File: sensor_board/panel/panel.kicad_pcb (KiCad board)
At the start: 2 copper layers, 102.6 x 93.3 mm, 165 parts, among them J1 Comm, J2 OUTPUT, J3 INPUT, J4 LDO_GND, J5 LDO_VCC, U1 INA228, U2 AMS1117/WL9005P3

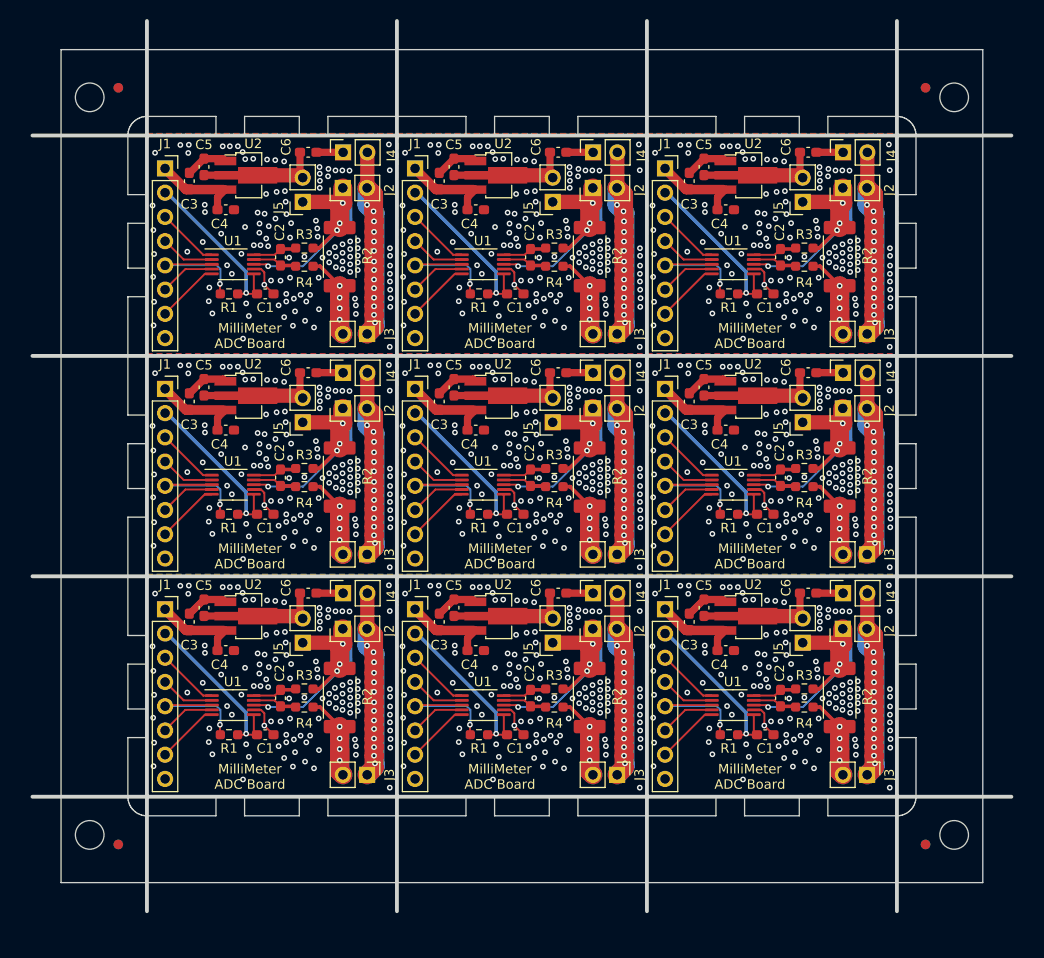
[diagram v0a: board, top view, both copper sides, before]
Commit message: Generate Rev. 1 gerber
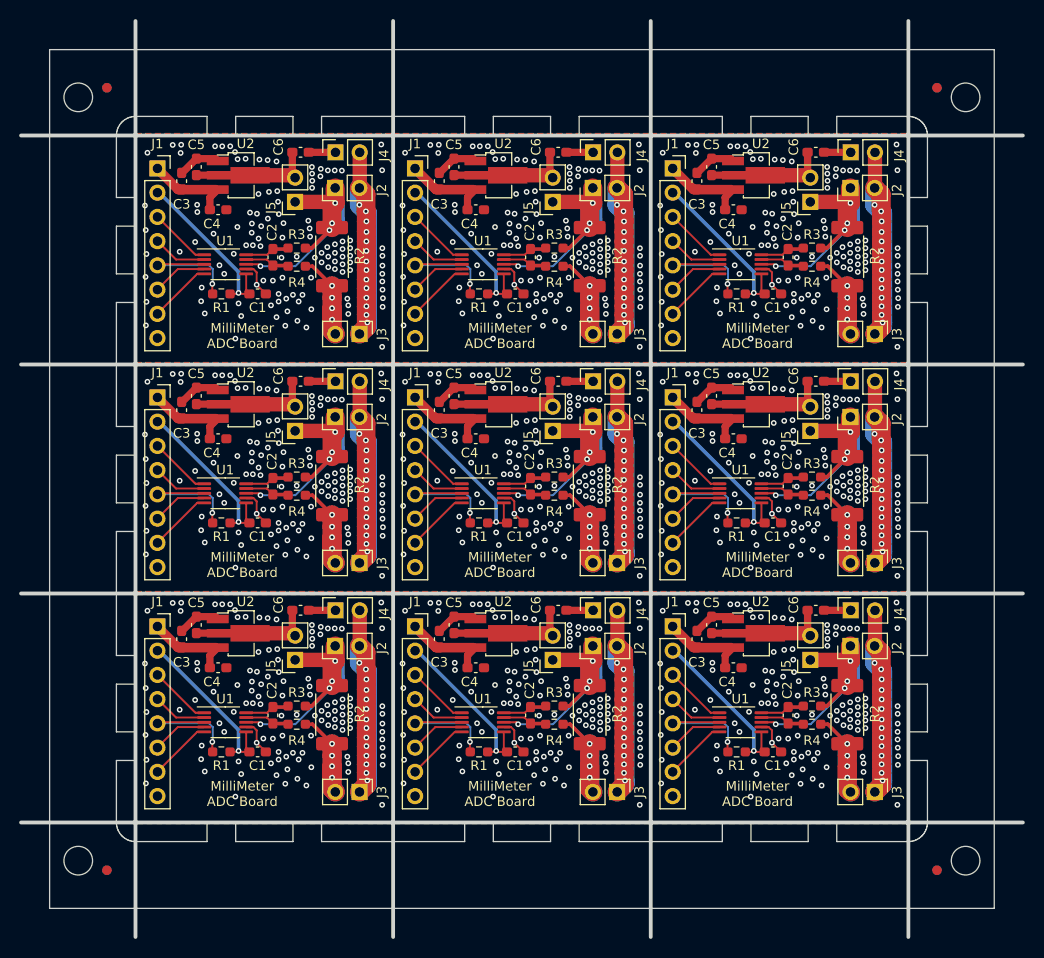
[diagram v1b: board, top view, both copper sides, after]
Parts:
- removed the C1 at (147.8, 68.7)
- removed the C1 at (121.6, 68.7)
- removed the C1 at (174.0, 91.8)
- removed the C1 at (174.0, 45.6)
- removed the C1 at (121.6, 91.8)
- removed the C1 at (121.6, 45.6)
- removed the C1 at (174.0, 68.7)
- removed the C1 at (147.8, 91.8)
- removed the C2 at (175.6, 88.0)
- removed the C2 at (149.4, 64.9)
- removed the C2 at (175.6, 41.8)
- removed the C2 at (175.6, 64.9)
- removed the C2 at (149.4, 88.0)
- removed the C2 at (123.2, 88.0)
- removed the C2 at (123.2, 64.9)
- removed the C2 at (123.2, 41.8)
- removed the C3 at (113.6, 80.0)
- removed the C3 at (139.8, 56.9)
- removed the C3 at (166.0, 56.9)
- removed the C3 at (113.6, 33.8)
- removed the C3 at (139.8, 80.0)
- removed the C3 at (166.0, 33.8)
- removed the C3 at (166.0, 80.0)
- removed the C3 at (113.6, 56.9)
- removed the C4 at (169.9, 59.9)
- removed the C4 at (143.7, 59.9)
- removed the C4 at (143.7, 83.0)
- removed the C4 at (117.5, 83.0)
- removed the C4 at (117.5, 59.9)
- removed the C4 at (117.5, 36.8)
- removed the C4 at (169.9, 36.8)
- removed the C4 at (169.9, 83.0)
- removed the C5 at (115.2, 78.5)
- removed the C5 at (167.6, 78.5)
- removed the C5 at (167.6, 55.4)
- removed the C5 at (141.4, 55.4)
- removed the C5 at (167.6, 32.3)
- removed the C5 at (141.4, 78.5)
- removed the C5 at (115.2, 32.3)
- removed the C5 at (115.2, 55.4)
- removed the C6 at (152.3, 53.9)
- removed the C6 at (178.5, 30.8)
- removed the C6 at (152.3, 77.0)
- removed the C6 at (178.5, 77.0)
- removed the C6 at (126.1, 77.0)
- removed the C6 at (126.1, 30.8)
- removed the C6 at (126.1, 53.9)
- removed the C6 at (178.5, 53.9)
- removed the J1 at (163.5, 78.7)
- removed the J1 at (111.1, 78.7)
- removed the J1 at (137.3, 78.7)
- removed the J1 at (137.3, 55.6)
- removed the J1 at (163.5, 55.6)
- removed the J1 at (111.1, 32.5)
- removed the J1 at (111.1, 55.6)
- removed the J1 at (163.5, 32.5)
- removed the J2 at (129.7, 80.7)
- removed the J2 at (182.1, 80.7)
- removed the J2 at (182.1, 57.6)
- removed the J2 at (155.9, 57.6)
- removed the J2 at (155.9, 80.7)
- removed the J2 at (129.7, 34.5)
- removed the J2 at (129.7, 57.6)
- removed the J2 at (182.1, 34.5)
- removed the J3 at (132.3, 72.9)
- removed the J3 at (184.7, 96.0)
- removed the J3 at (132.3, 96.0)
- removed the J3 at (132.3, 49.8)
- removed the J3 at (184.7, 72.9)
- removed the J3 at (158.5, 72.9)
- removed the J3 at (158.5, 96.0)
- removed the J3 at (184.7, 49.8)
- removed the J4 at (129.8, 53.9)
- removed the J4 at (182.2, 30.8)
- removed the J4 at (129.8, 77.0)
- removed the J4 at (129.8, 30.8)
- removed the J4 at (182.2, 77.0)
- removed the J4 at (156.0, 53.9)
- removed the J4 at (182.2, 53.9)
- removed the J4 at (156.0, 77.0)
- removed the J5 at (125.5, 82.2)
- removed the J5 at (125.5, 59.1)
- removed the J5 at (151.7, 82.2)
- removed the J5 at (177.9, 82.2)
- removed the J5 at (177.9, 36.0)
- removed the J5 at (151.7, 59.1)
- removed the J5 at (177.9, 59.1)
- removed the J5 at (125.5, 36.0)
- removed the R1 at (170.2, 91.8)
- removed the R1 at (117.8, 45.6)
- removed the R1 at (117.8, 68.7)
- removed the R1 at (117.8, 91.8)
- removed the R1 at (170.2, 68.7)
- removed the R1 at (170.2, 45.6)
- removed the R1 at (144.0, 91.8)
- removed the R1 at (144.0, 68.7)
- removed the R2 at (129.4, 41.7)
- removed the R2 at (181.8, 87.9)
- removed the R2 at (129.4, 87.9)
- removed the R2 at (181.8, 41.7)
- removed the R2 at (181.8, 64.8)
- removed the R2 at (155.6, 87.9)
- removed the R2 at (129.4, 64.8)
- removed the R2 at (155.6, 64.8)
- removed the R3 at (151.9, 87.0)
- removed the R3 at (125.7, 63.9)
- removed the R3 at (178.1, 40.8)
- removed the R3 at (178.1, 87.0)
- removed the R3 at (151.9, 63.9)
- removed the R3 at (178.1, 63.9)
- removed the R3 at (125.7, 87.0)
- removed the R3 at (125.7, 40.8)
- removed the R4 at (178.1, 88.9)
- removed the R4 at (125.7, 42.7)
- removed the R4 at (125.7, 88.9)
- removed the R4 at (151.9, 88.9)
- removed the R4 at (151.9, 65.8)
- removed the R4 at (178.1, 65.8)
- removed the R4 at (125.7, 65.8)
- removed the R4 at (178.1, 42.7)
- removed the REF** at (103.2, 25.0)
- removed the REF** at (106.2, 103.3) (x2)
- removed the REF** at (106.2, 24.0) (x2)
- removed the REF** at (190.8, 24.0) (x2)
- removed the REF** at (193.8, 102.3)
- removed the REF** at (193.8, 25.0)
- removed the REF** at (190.8, 103.3) (x2)
- removed the REF** at (103.2, 102.3)
- removed the U1 at (144.4, 65.6)
- removed the U1 at (118.2, 65.6)
- removed the U1 at (170.6, 42.5)
- removed the U1 at (170.6, 88.7)
- removed the U1 at (118.2, 88.7)
- removed the U1 at (118.2, 42.5)
- removed the U1 at (144.4, 88.7)
- removed the U1 at (170.6, 65.6)
- removed the U2 at (145.8, 56.3)
- removed the U2 at (172.0, 33.2)
- removed the U2 at (119.6, 56.3)
- removed the U2 at (145.8, 79.4)
- removed the U2 at (172.0, 56.3)
- removed the U2 at (119.6, 79.4)
- removed the U2 at (119.6, 33.2)
- removed the U2 at (172.0, 79.4)
- added C1: 100nF, Capacitor_SMD:C_0603_1608Metric_Pad1.08x0.95mm_HandSolder, F.Cu at (147.8, 69.6)
- added C1: 100nF, Capacitor_SMD:C_0603_1608Metric_Pad1.08x0.95mm_HandSolder, F.Cu at (147.8, 93.6)
- added C1: 100nF, Capacitor_SMD:C_0603_1608Metric_Pad1.08x0.95mm_HandSolder, F.Cu at (120.8, 45.6)
- added C1: 100nF, Capacitor_SMD:C_0603_1608Metric_Pad1.08x0.95mm_HandSolder, F.Cu at (174.8, 45.6)
- added C1: 100nF, Capacitor_SMD:C_0603_1608Metric_Pad1.08x0.95mm_HandSolder, F.Cu at (120.8, 93.6)
- added C1: 100nF, Capacitor_SMD:C_0603_1608Metric_Pad1.08x0.95mm_HandSolder, F.Cu at (174.8, 69.6)
- added C1: 100nF, Capacitor_SMD:C_0603_1608Metric_Pad1.08x0.95mm_HandSolder, F.Cu at (174.8, 93.6)
- added C1: 100nF, Capacitor_SMD:C_0603_1608Metric_Pad1.08x0.95mm_HandSolder, F.Cu at (120.8, 69.6)
- added C2: 100nF, Capacitor_SMD:C_0603_1608Metric_Pad1.08x0.95mm_HandSolder, F.Cu at (149.4, 65.8)
- added C2: 100nF, Capacitor_SMD:C_0603_1608Metric_Pad1.08x0.95mm_HandSolder, F.Cu at (176.4, 65.8)
- added C2: 100nF, Capacitor_SMD:C_0603_1608Metric_Pad1.08x0.95mm_HandSolder, F.Cu at (122.4, 41.8)
- added C2: 100nF, Capacitor_SMD:C_0603_1608Metric_Pad1.08x0.95mm_HandSolder, F.Cu at (122.4, 65.8)
- added C2: 100nF, Capacitor_SMD:C_0603_1608Metric_Pad1.08x0.95mm_HandSolder, F.Cu at (122.4, 89.8)
- added C2: 100nF, Capacitor_SMD:C_0603_1608Metric_Pad1.08x0.95mm_HandSolder, F.Cu at (176.4, 41.8)
- added C2: 100nF, Capacitor_SMD:C_0603_1608Metric_Pad1.08x0.95mm_HandSolder, F.Cu at (149.4, 89.8)
- added C2: 100nF, Capacitor_SMD:C_0603_1608Metric_Pad1.08x0.95mm_HandSolder, F.Cu at (176.4, 89.8)
- added C3: 10uF, Capacitor_SMD:C_0603_1608Metric_Pad1.08x0.95mm_HandSolder, F.Cu at (112.8, 57.8)
- added C3: 10uF, Capacitor_SMD:C_0603_1608Metric_Pad1.08x0.95mm_HandSolder, F.Cu at (166.8, 81.8)
- added C3: 10uF, Capacitor_SMD:C_0603_1608Metric_Pad1.08x0.95mm_HandSolder, F.Cu at (166.8, 33.8)
- added C3: 10uF, Capacitor_SMD:C_0603_1608Metric_Pad1.08x0.95mm_HandSolder, F.Cu at (166.8, 57.8)
- added C3: 10uF, Capacitor_SMD:C_0603_1608Metric_Pad1.08x0.95mm_HandSolder, F.Cu at (139.8, 81.8)
- added C3: 10uF, Capacitor_SMD:C_0603_1608Metric_Pad1.08x0.95mm_HandSolder, F.Cu at (112.8, 81.8)
- added C3: 10uF, Capacitor_SMD:C_0603_1608Metric_Pad1.08x0.95mm_HandSolder, F.Cu at (112.8, 33.8)
- added C3: 10uF, Capacitor_SMD:C_0603_1608Metric_Pad1.08x0.95mm_HandSolder, F.Cu at (139.8, 57.8)
- added C4: 0.1uF, Capacitor_SMD:C_0603_1608Metric_Pad1.08x0.95mm_HandSolder, F.Cu at (170.7, 36.8)
- added C4: 0.1uF, Capacitor_SMD:C_0603_1608Metric_Pad1.08x0.95mm_HandSolder, F.Cu at (170.7, 60.8)
- added C4: 0.1uF, Capacitor_SMD:C_0603_1608Metric_Pad1.08x0.95mm_HandSolder, F.Cu at (116.7, 36.8)
- added C4: 0.1uF, Capacitor_SMD:C_0603_1608Metric_Pad1.08x0.95mm_HandSolder, F.Cu at (143.7, 60.8)
- added C4: 0.1uF, Capacitor_SMD:C_0603_1608Metric_Pad1.08x0.95mm_HandSolder, F.Cu at (116.7, 60.8)
- added C4: 0.1uF, Capacitor_SMD:C_0603_1608Metric_Pad1.08x0.95mm_HandSolder, F.Cu at (143.7, 84.8)
- added C4: 0.1uF, Capacitor_SMD:C_0603_1608Metric_Pad1.08x0.95mm_HandSolder, F.Cu at (116.7, 84.8)
- added C4: 0.1uF, Capacitor_SMD:C_0603_1608Metric_Pad1.08x0.95mm_HandSolder, F.Cu at (170.7, 84.8)
- added C5: 0.1uF, Capacitor_SMD:C_0603_1608Metric_Pad1.08x0.95mm_HandSolder, F.Cu at (168.4, 80.3)
- added C5: 0.1uF, Capacitor_SMD:C_0603_1608Metric_Pad1.08x0.95mm_HandSolder, F.Cu at (114.4, 80.3)
- added C5: 0.1uF, Capacitor_SMD:C_0603_1608Metric_Pad1.08x0.95mm_HandSolder, F.Cu at (168.4, 56.3)
- added C5: 0.1uF, Capacitor_SMD:C_0603_1608Metric_Pad1.08x0.95mm_HandSolder, F.Cu at (141.4, 56.3)
- added C5: 0.1uF, Capacitor_SMD:C_0603_1608Metric_Pad1.08x0.95mm_HandSolder, F.Cu at (114.4, 56.3)
- added C5: 0.1uF, Capacitor_SMD:C_0603_1608Metric_Pad1.08x0.95mm_HandSolder, F.Cu at (168.4, 32.3)
- added C5: 0.1uF, Capacitor_SMD:C_0603_1608Metric_Pad1.08x0.95mm_HandSolder, F.Cu at (141.4, 80.3)
- added C5: 0.1uF, Capacitor_SMD:C_0603_1608Metric_Pad1.08x0.95mm_HandSolder, F.Cu at (114.4, 32.3)
- added C6: 10uF, Capacitor_SMD:C_0603_1608Metric_Pad1.08x0.95mm_HandSolder, F.Cu at (152.3, 54.8)
- added C6: 10uF, Capacitor_SMD:C_0603_1608Metric_Pad1.08x0.95mm_HandSolder, F.Cu at (125.3, 78.8)
- added C6: 10uF, Capacitor_SMD:C_0603_1608Metric_Pad1.08x0.95mm_HandSolder, F.Cu at (179.3, 78.8)
- added C6: 10uF, Capacitor_SMD:C_0603_1608Metric_Pad1.08x0.95mm_HandSolder, F.Cu at (152.3, 78.8)
- added C6: 10uF, Capacitor_SMD:C_0603_1608Metric_Pad1.08x0.95mm_HandSolder, F.Cu at (179.3, 30.8)
- added C6: 10uF, Capacitor_SMD:C_0603_1608Metric_Pad1.08x0.95mm_HandSolder, F.Cu at (125.3, 30.8)
- added C6: 10uF, Capacitor_SMD:C_0603_1608Metric_Pad1.08x0.95mm_HandSolder, F.Cu at (125.3, 54.8)
- added C6: 10uF, Capacitor_SMD:C_0603_1608Metric_Pad1.08x0.95mm_HandSolder, F.Cu at (179.3, 54.8)
- added J1: Comm, Connector_PinSocket_2.54mm:PinSocket_1x08_P2.54mm_Vertical, F.Cu at (137.3, 56.5)
- added J1: Comm, Connector_PinSocket_2.54mm:PinSocket_1x08_P2.54mm_Vertical, F.Cu at (110.3, 32.5)
- added J1: Comm, Connector_PinSocket_2.54mm:PinSocket_1x08_P2.54mm_Vertical, F.Cu at (110.3, 80.5)
- added J1: Comm, Connector_PinSocket_2.54mm:PinSocket_1x08_P2.54mm_Vertical, F.Cu at (110.3, 56.5)
- added J1: Comm, Connector_PinSocket_2.54mm:PinSocket_1x08_P2.54mm_Vertical, F.Cu at (164.3, 56.5)
- added J1: Comm, Connector_PinSocket_2.54mm:PinSocket_1x08_P2.54mm_Vertical, F.Cu at (137.3, 80.5)
- added J1: Comm, Connector_PinSocket_2.54mm:PinSocket_1x08_P2.54mm_Vertical, F.Cu at (164.3, 32.5)
- added J1: Comm, Connector_PinSocket_2.54mm:PinSocket_1x08_P2.54mm_Vertical, F.Cu at (164.3, 80.5)
- added J2: OUTPUT, Connector_PinHeader_2.54mm:PinHeader_1x02_P2.54mm_Vertical, F.Cu at (128.9, 82.5)
- added J2: OUTPUT, Connector_PinHeader_2.54mm:PinHeader_1x02_P2.54mm_Vertical, F.Cu at (182.9, 34.5)
- added J2: OUTPUT, Connector_PinHeader_2.54mm:PinHeader_1x02_P2.54mm_Vertical, F.Cu at (155.9, 82.5)
- added J2: OUTPUT, Connector_PinHeader_2.54mm:PinHeader_1x02_P2.54mm_Vertical, F.Cu at (182.9, 58.5)
- added J2: OUTPUT, Connector_PinHeader_2.54mm:PinHeader_1x02_P2.54mm_Vertical, F.Cu at (128.9, 58.5)
- added J2: OUTPUT, Connector_PinHeader_2.54mm:PinHeader_1x02_P2.54mm_Vertical, F.Cu at (182.9, 82.5)
- added J2: OUTPUT, Connector_PinHeader_2.54mm:PinHeader_1x02_P2.54mm_Vertical, F.Cu at (155.9, 58.5)
- added J2: OUTPUT, Connector_PinHeader_2.54mm:PinHeader_1x02_P2.54mm_Vertical, F.Cu at (128.9, 34.5)
- added J3: INPUT, Connector_PinHeader_2.54mm:PinHeader_1x02_P2.54mm_Vertical, F.Cu at (185.5, 97.8)
- added J3: INPUT, Connector_PinHeader_2.54mm:PinHeader_1x02_P2.54mm_Vertical, F.Cu at (158.5, 97.8)
- added J3: INPUT, Connector_PinHeader_2.54mm:PinHeader_1x02_P2.54mm_Vertical, F.Cu at (158.5, 73.8)
- added J3: INPUT, Connector_PinHeader_2.54mm:PinHeader_1x02_P2.54mm_Vertical, F.Cu at (185.5, 49.8)
- added J3: INPUT, Connector_PinHeader_2.54mm:PinHeader_1x02_P2.54mm_Vertical, F.Cu at (131.5, 73.8)
- added J3: INPUT, Connector_PinHeader_2.54mm:PinHeader_1x02_P2.54mm_Vertical, F.Cu at (185.5, 73.8)
- added J3: INPUT, Connector_PinHeader_2.54mm:PinHeader_1x02_P2.54mm_Vertical, F.Cu at (131.5, 97.8)
- added J3: INPUT, Connector_PinHeader_2.54mm:PinHeader_1x02_P2.54mm_Vertical, F.Cu at (131.5, 49.8)
- added J4: LDO_GND, Connector_PinSocket_2.54mm:PinSocket_1x02_P2.54mm_Vertical, F.Cu at (156.0, 54.8)
- added J4: LDO_GND, Connector_PinSocket_2.54mm:PinSocket_1x02_P2.54mm_Vertical, F.Cu at (183.0, 78.8)
- added J4: LDO_GND, Connector_PinSocket_2.54mm:PinSocket_1x02_P2.54mm_Vertical, F.Cu at (129.0, 54.8)
- added J4: LDO_GND, Connector_PinSocket_2.54mm:PinSocket_1x02_P2.54mm_Vertical, F.Cu at (129.0, 30.8)
- added J4: LDO_GND, Connector_PinSocket_2.54mm:PinSocket_1x02_P2.54mm_Vertical, F.Cu at (183.0, 54.8)
- added J4: LDO_GND, Connector_PinSocket_2.54mm:PinSocket_1x02_P2.54mm_Vertical, F.Cu at (156.0, 78.8)
- added J4: LDO_GND, Connector_PinSocket_2.54mm:PinSocket_1x02_P2.54mm_Vertical, F.Cu at (129.0, 78.8)
- added J4: LDO_GND, Connector_PinSocket_2.54mm:PinSocket_1x02_P2.54mm_Vertical, F.Cu at (183.0, 30.8)
- added J5: LDO_VCC, Connector_PinSocket_2.54mm:PinSocket_1x02_P2.54mm_Vertical, F.Cu at (151.7, 60.0)
- added J5: LDO_VCC, Connector_PinSocket_2.54mm:PinSocket_1x02_P2.54mm_Vertical, F.Cu at (124.7, 36.0)
- added J5: LDO_VCC, Connector_PinSocket_2.54mm:PinSocket_1x02_P2.54mm_Vertical, F.Cu at (178.7, 36.0)
- added J5: LDO_VCC, Connector_PinSocket_2.54mm:PinSocket_1x02_P2.54mm_Vertical, F.Cu at (124.7, 84.0)
- added J5: LDO_VCC, Connector_PinSocket_2.54mm:PinSocket_1x02_P2.54mm_Vertical, F.Cu at (151.7, 84.0)
- added J5: LDO_VCC, Connector_PinSocket_2.54mm:PinSocket_1x02_P2.54mm_Vertical, F.Cu at (178.7, 60.0)
- added J5: LDO_VCC, Connector_PinSocket_2.54mm:PinSocket_1x02_P2.54mm_Vertical, F.Cu at (178.7, 84.0)
- added J5: LDO_VCC, Connector_PinSocket_2.54mm:PinSocket_1x02_P2.54mm_Vertical, F.Cu at (124.7, 60.0)
- added R1: 10k, Resistor_SMD:R_0603_1608Metric_Pad0.98x0.95mm_HandSolder, F.Cu at (117.0, 93.6)
- added R1: 10k, Resistor_SMD:R_0603_1608Metric_Pad0.98x0.95mm_HandSolder, F.Cu at (171.0, 45.6)
- added R1: 10k, Resistor_SMD:R_0603_1608Metric_Pad0.98x0.95mm_HandSolder, F.Cu at (117.0, 45.6)
- added R1: 10k, Resistor_SMD:R_0603_1608Metric_Pad0.98x0.95mm_HandSolder, F.Cu at (144.0, 69.6)
- added R1: 10k, Resistor_SMD:R_0603_1608Metric_Pad0.98x0.95mm_HandSolder, F.Cu at (171.0, 93.6)
- added R1: 10k, Resistor_SMD:R_0603_1608Metric_Pad0.98x0.95mm_HandSolder, F.Cu at (171.0, 69.6)
- added R1: 10k, Resistor_SMD:R_0603_1608Metric_Pad0.98x0.95mm_HandSolder, F.Cu at (144.0, 93.6)
- added R1: 10k, Resistor_SMD:R_0603_1608Metric_Pad0.98x0.95mm_HandSolder, F.Cu at (117.0, 69.6)
- added R2: 0.05R, Resistor_SMD:R_2512_6332Metric_Pad1.40x3.35mm_HandSolder, F.Cu at (182.6, 89.7)
- added R2: 0.05R, Resistor_SMD:R_2512_6332Metric_Pad1.40x3.35mm_HandSolder, F.Cu at (182.6, 65.7)
- added R2: 0.05R, Resistor_SMD:R_2512_6332Metric_Pad1.40x3.35mm_HandSolder, F.Cu at (128.6, 89.7)
- added R2: 0.05R, Resistor_SMD:R_2512_6332Metric_Pad1.40x3.35mm_HandSolder, F.Cu at (128.6, 41.7)
- added R2: 0.05R, Resistor_SMD:R_2512_6332Metric_Pad1.40x3.35mm_HandSolder, F.Cu at (155.6, 89.7)
- added R2: 0.05R, Resistor_SMD:R_2512_6332Metric_Pad1.40x3.35mm_HandSolder, F.Cu at (155.6, 65.7)
- added R2: 0.05R, Resistor_SMD:R_2512_6332Metric_Pad1.40x3.35mm_HandSolder, F.Cu at (128.6, 65.7)
- added R2: 0.05R, Resistor_SMD:R_2512_6332Metric_Pad1.40x3.35mm_HandSolder, F.Cu at (182.6, 41.7)
- added R3: 47R, Resistor_SMD:R_0603_1608Metric_Pad0.98x0.95mm_HandSolder, F.Cu at (151.9, 64.8)
- added R3: 47R, Resistor_SMD:R_0603_1608Metric_Pad0.98x0.95mm_HandSolder, F.Cu at (124.9, 64.8)
- added R3: 47R, Resistor_SMD:R_0603_1608Metric_Pad0.98x0.95mm_HandSolder, F.Cu at (151.9, 88.8)
- added R3: 47R, Resistor_SMD:R_0603_1608Metric_Pad0.98x0.95mm_HandSolder, F.Cu at (178.9, 40.8)
- added R3: 47R, Resistor_SMD:R_0603_1608Metric_Pad0.98x0.95mm_HandSolder, F.Cu at (124.9, 88.8)
- added R3: 47R, Resistor_SMD:R_0603_1608Metric_Pad0.98x0.95mm_HandSolder, F.Cu at (178.9, 64.8)
- added R3: 47R, Resistor_SMD:R_0603_1608Metric_Pad0.98x0.95mm_HandSolder, F.Cu at (178.9, 88.8)
- added R3: 47R, Resistor_SMD:R_0603_1608Metric_Pad0.98x0.95mm_HandSolder, F.Cu at (124.9, 40.8)
- added R4: 47R, Resistor_SMD:R_0603_1608Metric_Pad0.98x0.95mm_HandSolder, F.Cu at (178.9, 90.7)
- added R4: 47R, Resistor_SMD:R_0603_1608Metric_Pad0.98x0.95mm_HandSolder, F.Cu at (151.9, 90.7)
- added R4: 47R, Resistor_SMD:R_0603_1608Metric_Pad0.98x0.95mm_HandSolder, F.Cu at (151.9, 66.7)
- added R4: 47R, Resistor_SMD:R_0603_1608Metric_Pad0.98x0.95mm_HandSolder, F.Cu at (124.9, 66.7)
- added R4: 47R, Resistor_SMD:R_0603_1608Metric_Pad0.98x0.95mm_HandSolder, F.Cu at (178.9, 66.7)
- added R4: 47R, Resistor_SMD:R_0603_1608Metric_Pad0.98x0.95mm_HandSolder, F.Cu at (124.9, 42.7)
- added R4: 47R, Resistor_SMD:R_0603_1608Metric_Pad0.98x0.95mm_HandSolder, F.Cu at (178.9, 42.7)
- added R4: 47R, Resistor_SMD:R_0603_1608Metric_Pad0.98x0.95mm_HandSolder, F.Cu at (124.9, 90.7)
- added REF**: NPTH, NPTH, F.Cu at (195.0, 105.0)
- added REF**: Fiducial, Fiducial, B.Cu at (105.0, 24.0)
- added REF**: Fiducial, Fiducial, B.Cu at (192.0, 106.0)
- added REF**: Fiducial, Fiducial, B.Cu at (105.0, 106.0)
- added REF**: NPTH, NPTH, F.Cu at (195.0, 25.0)
- added REF**: Fiducial, Fiducial, F.Cu at (192.0, 106.0)
- added REF**: NPTH, NPTH, F.Cu at (102.0, 25.0)
- added REF**: Fiducial, Fiducial, F.Cu at (105.0, 106.0)
- added REF**: Fiducial, Fiducial, F.Cu at (192.0, 24.0)
- added REF**: NPTH, NPTH, F.Cu at (102.0, 105.0)
- added REF**: Fiducial, Fiducial, F.Cu at (105.0, 24.0)
- added REF**: Fiducial, Fiducial, B.Cu at (192.0, 24.0)
- added U1: INA228, Package_SO:VSSOP-10_3x3mm_P0.5mm, F.Cu at (117.4, 42.5)
- added U1: INA228, Package_SO:VSSOP-10_3x3mm_P0.5mm, F.Cu at (144.4, 66.5)
- added U1: INA228, Package_SO:VSSOP-10_3x3mm_P0.5mm, F.Cu at (171.4, 42.5)
- added U1: INA228, Package_SO:VSSOP-10_3x3mm_P0.5mm, F.Cu at (117.4, 66.5)
- added U1: INA228, Package_SO:VSSOP-10_3x3mm_P0.5mm, F.Cu at (144.4, 90.5)
- added U1: INA228, Package_SO:VSSOP-10_3x3mm_P0.5mm, F.Cu at (171.4, 66.5)
- added U1: INA228, Package_SO:VSSOP-10_3x3mm_P0.5mm, F.Cu at (171.4, 90.5)
- added U1: INA228, Package_SO:VSSOP-10_3x3mm_P0.5mm, F.Cu at (117.4, 90.5)
- added U2: AMS1117/WL9005P3, Package_TO_SOT_SMD:SOT-89-3_Handsoldering, F.Cu at (172.8, 33.2)
- added U2: AMS1117/WL9005P3, Package_TO_SOT_SMD:SOT-89-3_Handsoldering, F.Cu at (172.8, 81.2)
- added U2: AMS1117/WL9005P3, Package_TO_SOT_SMD:SOT-89-3_Handsoldering, F.Cu at (118.8, 57.2)
- added U2: AMS1117/WL9005P3, Package_TO_SOT_SMD:SOT-89-3_Handsoldering, F.Cu at (118.8, 33.2)
- added U2: AMS1117/WL9005P3, Package_TO_SOT_SMD:SOT-89-3_Handsoldering, F.Cu at (118.8, 81.2)
- added U2: AMS1117/WL9005P3, Package_TO_SOT_SMD:SOT-89-3_Handsoldering, F.Cu at (145.8, 81.2)
- added U2: AMS1117/WL9005P3, Package_TO_SOT_SMD:SOT-89-3_Handsoldering, F.Cu at (172.8, 57.2)
- added U2: AMS1117/WL9005P3, Package_TO_SOT_SMD:SOT-89-3_Handsoldering, F.Cu at (145.8, 57.2)
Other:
- board size 102.6 x 93.3 mm -> 105 x 96 mm
